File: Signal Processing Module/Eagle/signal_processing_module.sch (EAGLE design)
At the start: 26 parts, among them IC1 LM324N, IC2 TL061P

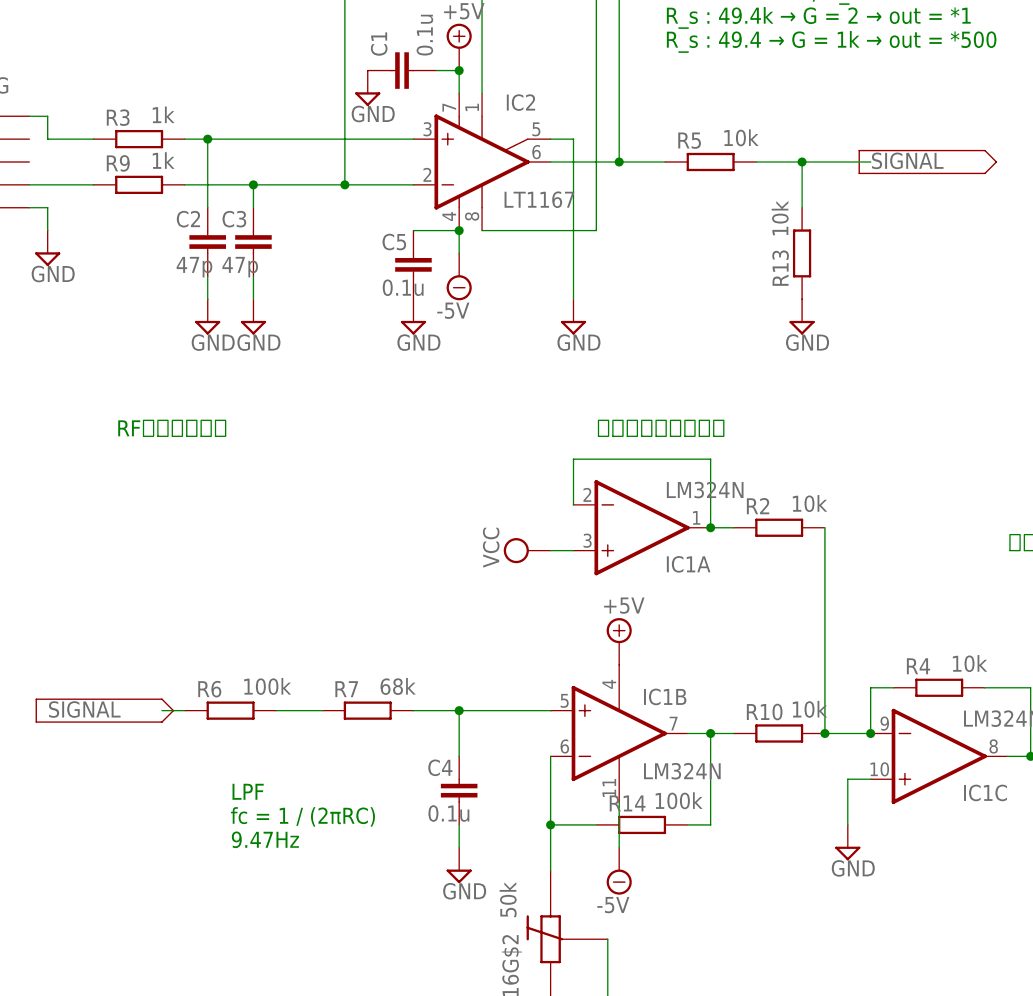
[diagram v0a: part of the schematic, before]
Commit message: Update: v1.1.0
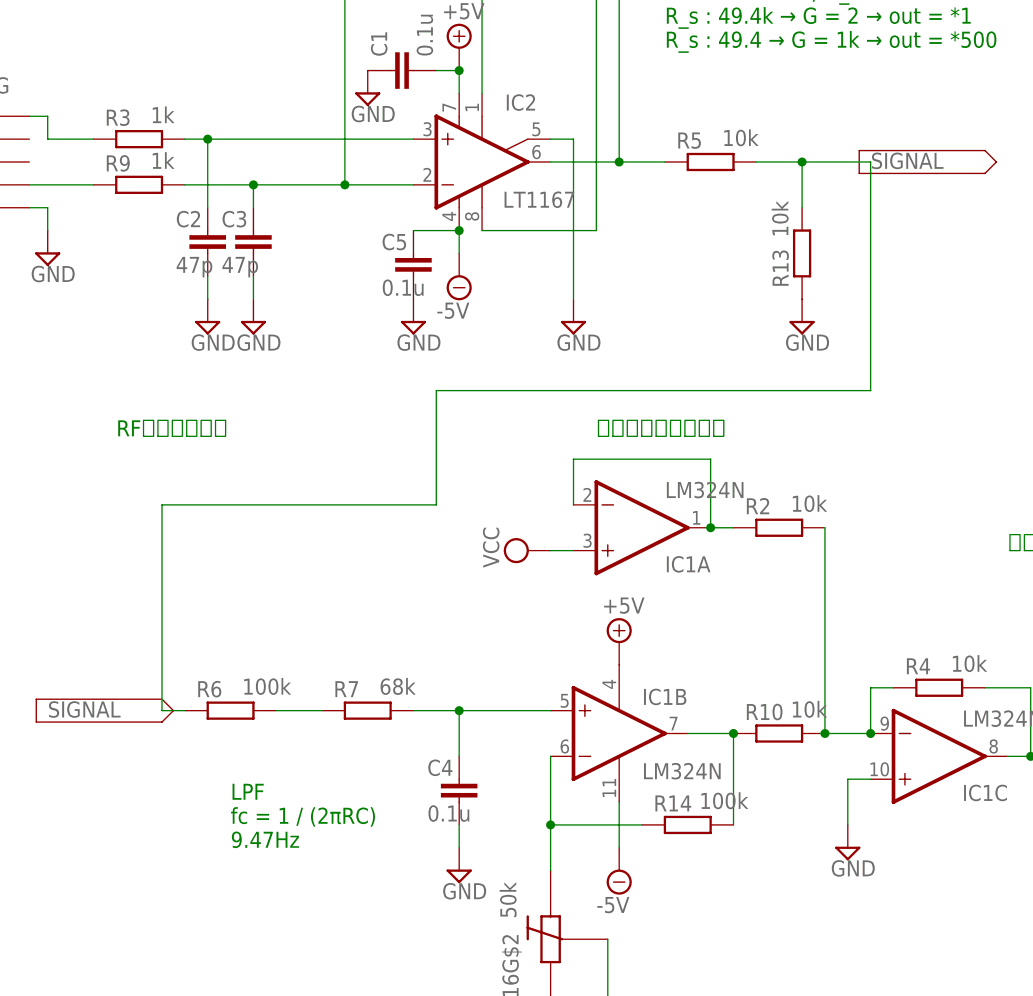
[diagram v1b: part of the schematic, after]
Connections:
- removed net N$16: R13.2, R5.2
- net N$17: now also R13.2, R5.2
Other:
- moved on the sheet: R14
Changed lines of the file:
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@@
 </instance>
 <instance part="IC1" gate="P" x="96.52" y="66.04" smashed="yes"/>
-<instance part="R14" gate="G$1" x="99.06" y="55.88" smashed="yes">
-<attribute name="NAME" x="95.25" y="57.3786" size="1.778" layer="95"/>
-<attribute name="VALUE" x="100.33" y="57.658" size="1.778" layer="96"/>
+<instance part="R14" gate="G$1" x="104.14" y="55.88" smashed="yes">
+<attribute name="NAME" x="100.33" y="57.3786" size="1.778" layer="95"/>
+<attribute name="VALUE" x="105.41" y="57.658" size="1.778" layer="96"/>
 </instance>
 <instance part="R16" gate="G$2" x="88.9" y="43.18" smashed="yes" rot="R90">
@@
 <net name="RAW_SIGNAL" class="0">
 <segment>
-<wire x1="106.68" y1="66.04" x2="106.68" y2="55.88" width="0.1524" layer="91"/>
-<wire x1="104.14" y1="66.04" x2="106.68" y2="66.04" width="0.1524" layer="91"/>
-<junction x="106.68" y="66.04"/>
-<wire x1="106.68" y1="66.04" x2="109.22" y2="66.04" width="0.1524" layer="91"/>
+<wire x1="109.22" y1="66.04" x2="109.22" y2="55.88" width="0.1524" layer="91"/>
+<wire x1="104.14" y1="66.04" x2="109.22" y2="66.04" width="0.1524" layer="91"/>
+<junction x="109.22" y="66.04"/>
 <pinref part="R10" gate="G$1" pin="1"/>
 <pinref part="IC1" gate="B" pin="OUT"/>
-<wire x1="104.14" y1="55.88" x2="106.68" y2="55.88" width="0.1524" layer="91"/>
 <pinref part="R14" gate="G$1" pin="2"/>
 </segment>
@@
 <wire x1="88.9" y1="86.36" x2="91.44" y2="86.36" width="0.1524" layer="91"/>
 <pinref part="IC1" gate="A" pin="+IN"/>
-</segment>
-</net>
-<net name="N$16" class="0">
-<segment>
-<pinref part="R5" gate="G$1" pin="2"/>
-<wire x1="111.76" y1="129.54" x2="116.84" y2="129.54" width="0.1524" layer="91"/>
-<pinref part="R13" gate="G$1" pin="2"/>
-<wire x1="116.84" y1="124.46" x2="116.84" y2="129.54" width="0.1524" layer="91"/>
-<junction x="116.84" y="129.54"/>
-<wire x1="124.46" y1="129.54" x2="116.84" y2="129.54" width="0.1524" layer="91"/>
 </segment>
 </net>
@@
 <pinref part="IC1" gate="B" pin="-IN"/>
 <wire x1="88.9" y1="63.5" x2="88.9" y2="55.88" width="0.1524" layer="91"/>
-<wire x1="88.9" y1="55.88" x2="93.98" y2="55.88" width="0.1524" layer="91"/>
+<wire x1="88.9" y1="55.88" x2="99.06" y2="55.88" width="0.1524" layer="91"/>
 <pinref part="R14" gate="G$1" pin="1"/>
 <pinref part="R16" gate="G$2" pin="P$3"/>
@@
 <pinref part="R6" gate="G$1" pin="1"/>
 <wire x1="45.72" y1="68.58" x2="48.26" y2="68.58" width="0.1524" layer="91"/>
+<wire x1="45.72" y1="68.58" x2="45.72" y2="91.44" width="0.1524" layer="91"/>
+<wire x1="45.72" y1="91.44" x2="76.2" y2="91.44" width="0.1524" layer="91"/>
+<wire x1="76.2" y1="91.44" x2="76.2" y2="104.14" width="0.1524" layer="91"/>
+<wire x1="76.2" y1="104.14" x2="124.46" y2="104.14" width="0.1524" layer="91"/>
+<pinref part="R5" gate="G$1" pin="2"/>
+<wire x1="111.76" y1="129.54" x2="116.84" y2="129.54" width="0.1524" layer="91"/>
+<pinref part="R13" gate="G$1" pin="2"/>
+<wire x1="116.84" y1="124.46" x2="116.84" y2="129.54" width="0.1524" layer="91"/>
+<junction x="116.84" y="129.54"/>
+<wire x1="124.46" y1="129.54" x2="116.84" y2="129.54" width="0.1524" layer="91"/>
+<wire x1="124.46" y1="104.14" x2="124.46" y2="129.54" width="0.1524" layer="91"/>
 </segment>
 </net>
@@
 </sheet>
 </sheets>
+<errors>
+</errors>
 </schematic>
 </drawing>
